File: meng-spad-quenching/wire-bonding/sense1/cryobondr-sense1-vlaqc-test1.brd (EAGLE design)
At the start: 46 x 46 mm, 30 parts, among them IC2 SENSE1, U1 SN74LVC1G34DBVT, X1 SPAD1, X10 AQCR3_VDD2V5, X11 HTR1, X12 HTR2, X2 SPAD2, X3 HTR3, X4 AQCR3_AV_DET, X5 AQCR3_IBIAS, X6 SPAD4, X7 SPAD3, X8 HTR4, X9 AQCR3_SPAD_CATHODE

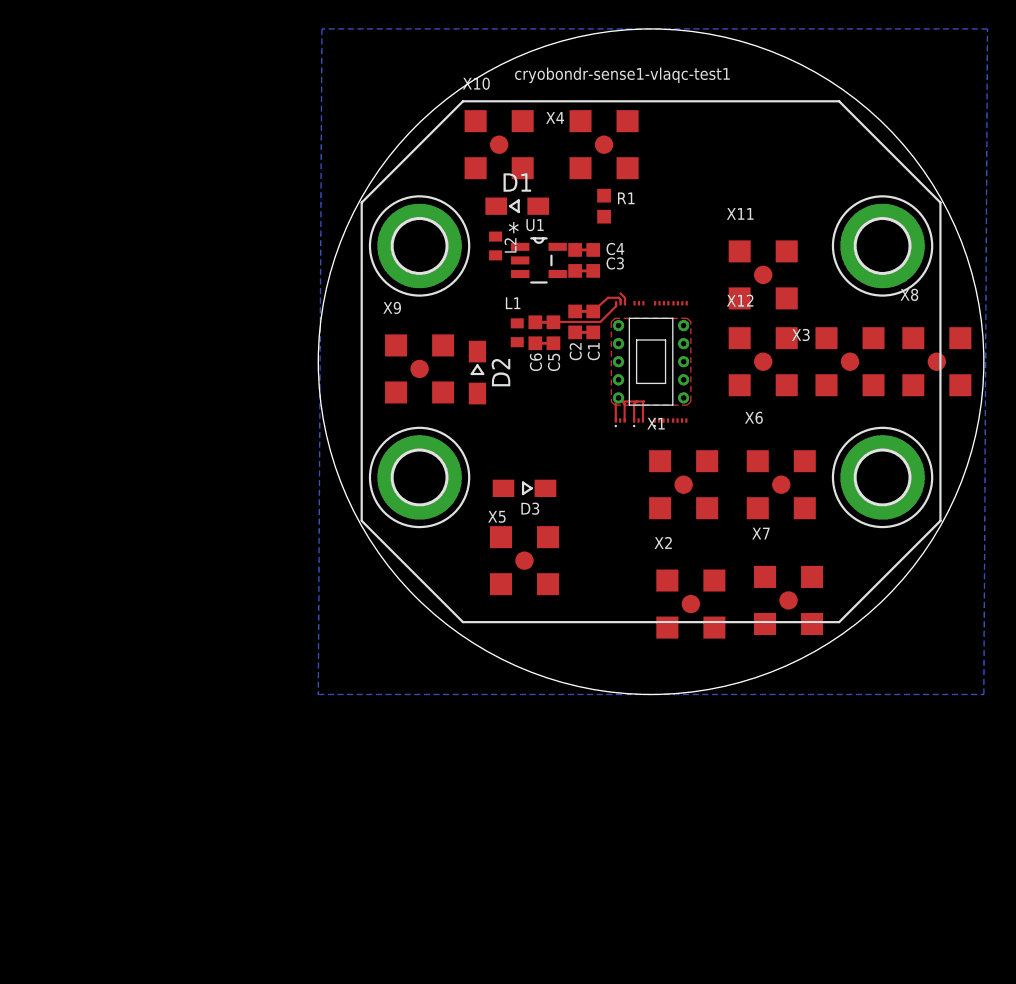
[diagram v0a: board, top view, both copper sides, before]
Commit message: Layout done, exported first gerber
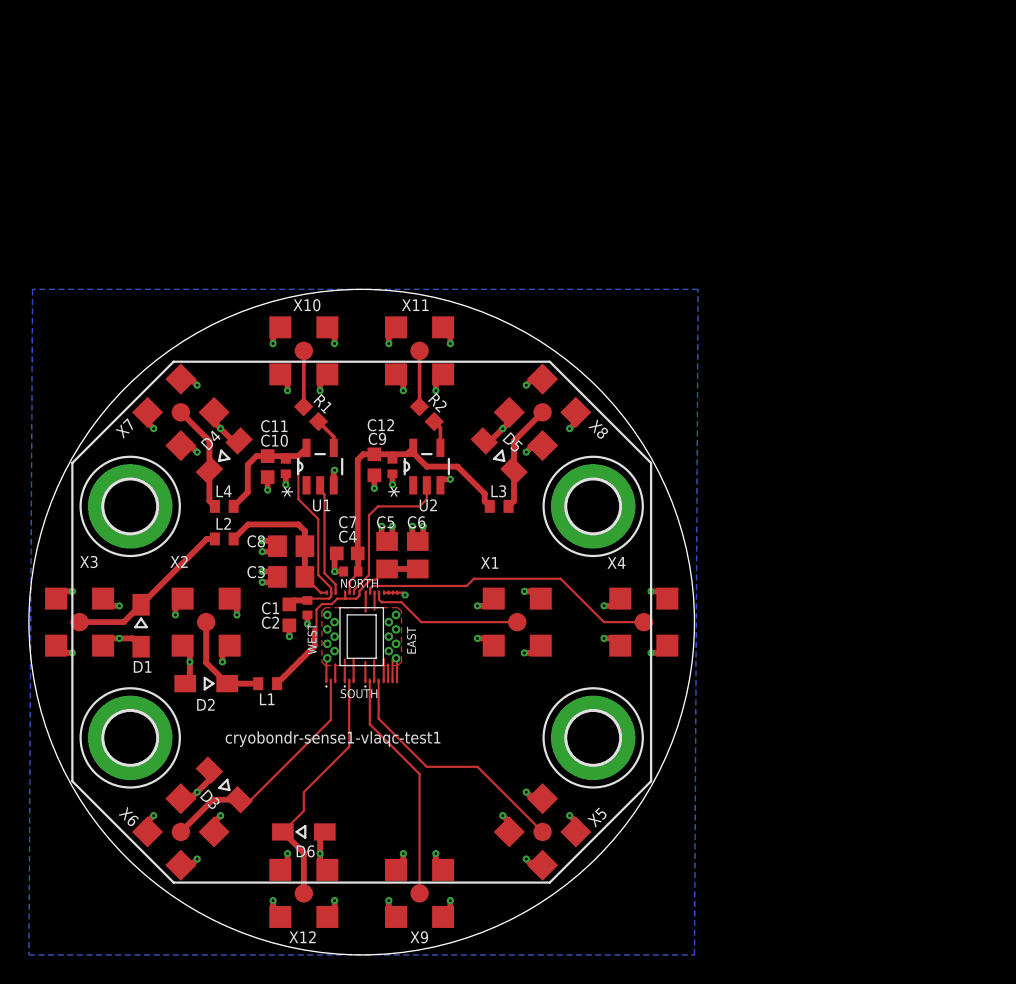
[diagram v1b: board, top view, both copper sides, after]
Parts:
- removed IC2: SENSE1, meng:SENSE1-WIREBOND-VLAQC-TEST1
- added C10, C9: IPDiA 935131424510, rcl-modified-footprints:C0402
- added C11, C12, C7: IPDiA 935131425610, rcl-modified-footprints:C0603
- added C8: ECH-U1C103JB5, rcl-modified-footprints:C0805
- added D4, D5, D6: UCLAMP3301D.TCT, diode:SOD323-W
- added IC1: SENSE1, meng:SENSE1-WIREBOND-VLAQC-TEST1
- added L3, L4: Samsung CIM05J152NC, meng:R0402
- added R2: Vishay FC0603E50R0BTBST1, rcl-modified-footprints:R0603
- added U2: SN74LVC1G34DBVT, Texas Instruments_By_element14_Batch_1:SOT95P280X145-5N
- C1: value 10n -> IPDiA 935131425610
- C2, C4: value 100n -> IPDiA 935131424510; device rcl-modified-footprints:C0603 -> rcl-modified-footprints:C0402
- C3: value 1u -> ECP-U1C104MA5; device rcl-modified-footprints:C0603 -> rcl-modified-footprints:C0805
- C5: value 100n -> ECP-U1C104MA5; device rcl-modified-footprints:C0603 -> rcl-modified-footprints:C0805
- C6: value 10n -> ECH-U1C103JB5; device rcl-modified-footprints:C0603 -> rcl-modified-footprints:C0805
- D1, D2: value (none) -> DF2B36FU,H3F
- D3: value (none) -> UCLAMP3301D.TCT
- L1, L2: value CHOKE_0402 -> Samsung CIM05J152NC
- R1: value 49R9 -> Vishay FC0603E50R0BTBST1
- X1: value SPAD1 -> HTR2
- X10: value AQCR3_VDD2V5 -> R3_OUT
- X11: value HTR1 -> R4_OUT
- X12: value HTR2 -> R4_IBIAS
- X2: value SPAD2 -> R4_VA
- X3: value HTR3 -> R3_VA
- X4: value AQCR3_AV_DET -> HTR1
- X5: value AQCR3_IBIAS -> SPAD2
- X6: value SPAD4 -> R3_IBIAS
- X7: value SPAD3 -> R3_2V5
- X8: value HTR4 -> R4_2V5
- X9: value AQCR3_SPAD_CATHODE -> SPAD1
- moved X3 56.2 mm to (-19.5, 0.00)
- moved X12 48.6 mm to (-4.00, -18.8)
- moved X6 47.9 mm to (-12.5, -14.5), turned to 45 degrees
- moved X7 44.0 mm to (-12.5, 14.5), turned to 45 degrees
- moved D1 38.9 mm to (-15.2, -0.25), turned to 270 degrees
- moved X9 36.2 mm to (4.00, -18.8)
- moved X2 33.5 mm to (-10.8, 0.00)
- moved X4 33.1 mm to (19.5, 0.00)
- moved C3 30.2 mm to (-4.88, 3.12), turned to 180 degrees
- moved L1 29.8 mm to (-6.50, -4.25), turned to 180 degrees
- moved C1 29.2 mm to (-5.00, 0.50)
- moved D3 29.2 mm to (-9.50, -11.2), turned to 135 degrees
- moved D2 28.5 mm to (-10.8, -4.25), turned to 180 degrees
- moved L2 27.6 mm to (-9.50, 5.75), turned to 180 degrees
- moved X8 27.5 mm to (12.5, 14.5), turned to 45 degrees
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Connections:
- net N$2 renamed R3_Y
- removed net N$1: D1.C, L2.1, X10.S
- removed net N$10: IC2.SPAD4_CATHODE, X6.S
- removed net N$11: IC2.SPAD4_ANODE, X6.G1, X6.G2, X6.G3, X6.G4
- removed net N$12: IC2.SPAD3_ANODE, X7.G1, X7.G2, X7.G3, X7.G4
- removed net N$13: IC2.SPAD3_CATHODE, X7.S
- removed net N$14: IC2.SPAD3_HEATER2, X3.S
- removed net N$15: IC2.SPAD4_HEATER2, X8.S
- removed net N$16: IC2.SPAD3_HEATER1, X3.G1, X3.G2, X3.G3, X3.G4
- removed net N$17: IC2.SPAD4_HEATER1, X8.G1, X8.G2, X8.G3, X8.G4
- removed net N$18: IC2.SPAD2_CATHODE, X2.S
- removed net N$19: IC2.SPAD2_ANODE, X2.G1, X2.G2, X2.G3, X2.G4
- removed net N$20: IC2.SPAD1_ANODE, X1.G1, X1.G2, X1.G3, X1.G4
- removed net N$21: IC2.SPAD1_CATHODE, X1.S
- removed net N$22: IC2.SPAD1_HEATER2, X11.S
- removed net N$23: IC2.SPAD2_HEATER2, X12.S
- removed net N$24: IC2.SPAD1_HEATER1, X11.G1, X11.G2, X11.G3, X11.G4
- removed net N$25: IC2.SPAD2_HEATER1, X12.G1, X12.G2, X12.G3, X12.G4
- removed net N$3: R1.2, X4.S
- removed net N$4: D3.C, IC2.AQCR3_HOLDOFF_IBIAS, X5.S
- removed net N$5: IC2.AQCR4_HOLDOFF_IBIAS
- removed net N$6: D2.C, L1.2, X9.S
- removed net N$7: IC2.AQCR3_AV_DET, U1.2
- new net AQCR3_AV_DET: IC1.AQCR3_AV_DET, U1.2
- new net AQCR3_IBIAS: D3.C, IC1.AQCR3_HOLDOFF_IBIAS, X6.S
- new net AQCR3_VA: D1.C, L2.2, X3.S
- new net AQCR3_VDD: D4.C, L4.1, X7.S
- new net AQCR4_AV_DET: IC1.AQCR4_AV_DET, U2.2
- new net AQCR4_IBIAS: D6.C, IC1.AQCR4_HOLDOFF_IBIAS, X12.S
- new net AQCR4_VA: D2.C, L1.2, X2.S
- new net AQCR4_VA_FILT: C5.1, C6.1, IC1.AQCR4_SPAD_CATHODE, L1.1
- new net AQCR4_VDD: D5.C, L3.1, X8.S
- new net AQCR4_VDD_FILT: C12.1, C4.1, C7.1, C9.1, IC1.AQCR4_VDD2V5, L3.2, U2.5
- new net R3_Y_R: R1.2, X10.S
- new net R4_Y: R2.1, U2.4
- new net R4_Y_R: R2.2, X11.S
- new net SPAD1_CATH: IC1.SPAD1_CATHODE, X9.S
- new net SPAD1_HTR: IC1.SPAD1_HEATER2, X4.S
- new net SPAD2_CATH: IC1.SPAD2_CATHODE, X5.S
- new net SPAD2_HTR: IC1.SPAD2_HEATER2, X1.S
- net AQCR3_VA_FILT: now also C3.1, C8.1, IC1.AQCR3_SPAD_CATHODE, L2.1; no longer C5.1, C6.1, IC2.AQCR3_SPAD_CATHODE, L1.1
- net AQCR3_VDD_FILT: now also C10.1, C11.1, IC1.AQCR3_VDD2V5, L4.2; no longer C3.1, C4.1, IC2.AQCR3_VDD2V5, L2.2
- net GND: now also C10.2, C11.2, C12.2, C7.2, C8.2, C9.2, D4.A, D5.A, D6.A, IC1.AQCR3_GND, IC1.AQCR3_GUARD_RING, IC1.AQCR4_GND, IC1.AQCR4_GUARD_RING, IC1.SPAD1_ANODE, IC1.SPAD1_HEATER1, IC1.SPAD2_ANODE, IC1.SPAD2_HEATER1, IC1.SPAD3_ANODE, IC1.SPAD3_CATHODE, IC1.SPAD3_HEATER1, IC1.SPAD3_HEATER2, IC1.SPAD4_ANODE, IC1.SPAD4_CATHODE, IC1.SPAD4_HEATER1, IC1.SPAD4_HEATER2, U2.3, X1.G1, X1.G2, X1.G3, X1.G4, X11.G1, X11.G2, X11.G3, X11.G4, X12.G1, X12.G2, X12.G3, X12.G4, X2.G1, X2.G2, X2.G3, X2.G4, X3.G1, X3.G2, X3.G3, X3.G4, X6.G1, X6.G2, X6.G3, X6.G4, X7.G1, X7.G2, X7.G3, X7.G4, X8.G1, X8.G2, X8.G3, X8.G4; no longer IC2.AQCR3_GND, IC2.AQCR3_GUARD_RING, IC2.AQCR4_GND, IC2.AQCR4_GUARD_RING
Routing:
- net GND: track 11.4 -> 109.9 mm, vias 10 -> 80
- net AQCR4_VDD_FILT: track 0.00 -> 21.4 mm
- net SPAD1_HTR: track 0.00 -> 20.7 mm
- net AQCR4_IBIAS: track 0.00 -> 17.2 mm
- net SPAD2_CATH: track 0.00 -> 17.2 mm
- net AQCR3_VDD_FILT: track 5.06 -> 21.8 mm
- net AQCR3_IBIAS: track 0.00 -> 16.3 mm
- net SPAD1_CATH: track 0.00 -> 16.1 mm
- net AQCR4_VA_FILT: track 0.00 -> 15.3 mm
- net AQCR3_VA: track 0.00 -> 11.7 mm
- net AQCR4_AV_DET: track 0.00 -> 11.2 mm
- net SPAD2_HTR: track 0.00 -> 10.7 mm
- net AQCR3_AV_DET: track 0.00 -> 7.86 mm
- net AQCR3_VDD: track 0.00 -> 7.62 mm
- net AQCR4_VDD: track 0.00 -> 7.47 mm
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- added copper zone on layer 1, net AQCR4_VA_FILT
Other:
- board text added: "EAST"
- board text added: "NORTH"
- board text added: "SOUTH"
- board text added: "WEST"
